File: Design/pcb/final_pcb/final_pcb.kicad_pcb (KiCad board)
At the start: 2 copper layers, 86.5 x 42 mm, 42 parts, among them J1 USB_C_Receptacle_USB2.0_14P, J2 Screw_Terminal_01x02, J3 Screw_Terminal_01x02, J5 Conn_01x05_Pin, Q1 NMOS, Q2 NMOS, U1 IR2184, U2 PIC32MZ2048EFM144-I/PH, U3 LM7812, U5 TPS560200, Y1 SG-8002CA

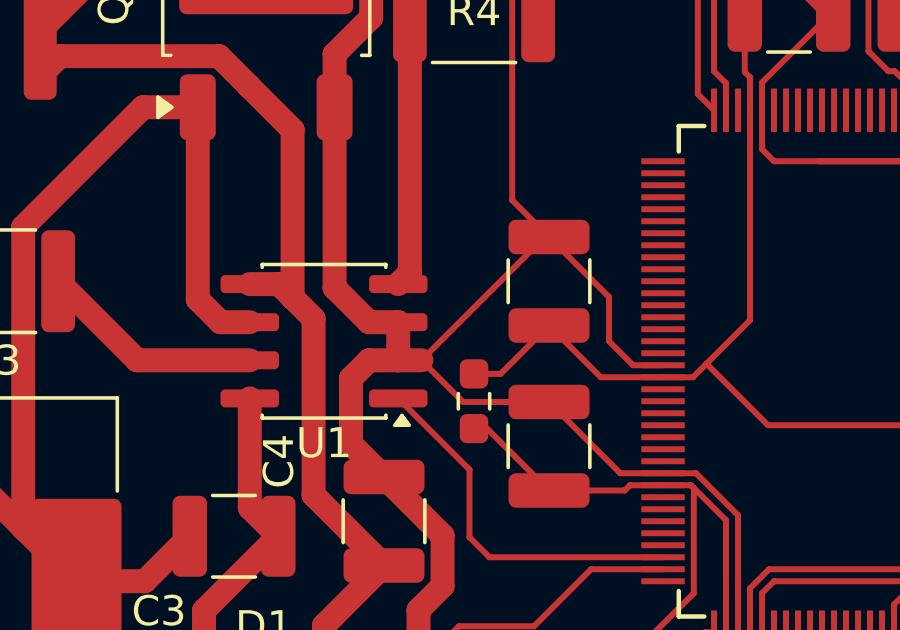
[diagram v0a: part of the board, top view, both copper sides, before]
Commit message: pcb fix
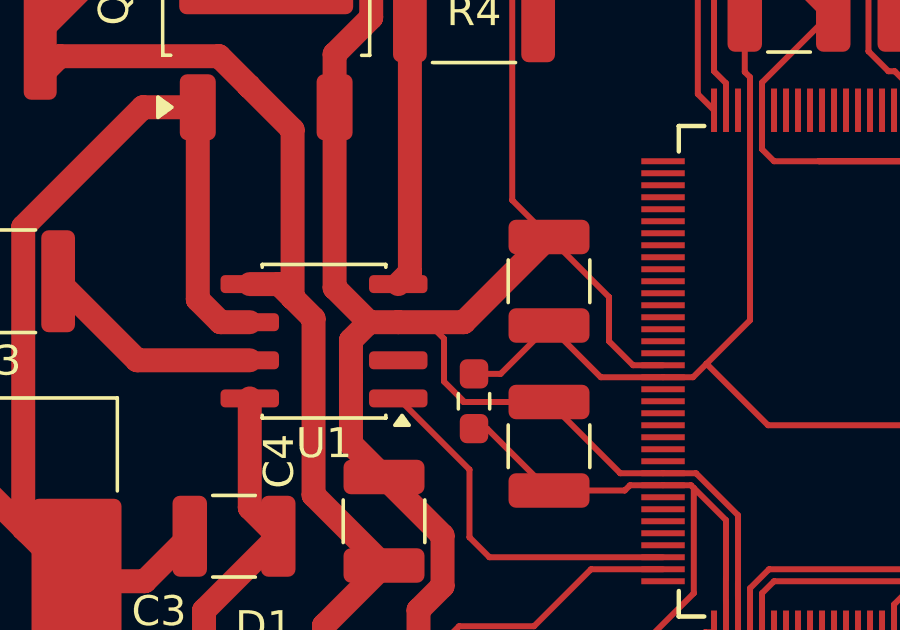
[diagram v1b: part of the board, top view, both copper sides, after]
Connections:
- U1 pad 2: GND -> unconnected-(U1-~{SD}-Pad2)
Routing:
- net GND: track 453.0 -> 454.1 mm
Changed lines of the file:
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@@
 	(net 143 "Net-(U5-FB)")
 	(net 144 "Net-(U5-PH)")
+	(net 145 "unconnected-(U1-~{SD}-Pad2)")
 	(footprint "Capacitor_SMD:C_1210_3225Metric"
 		(layer "F.Cu")
@@
 			(layers "F.Cu" "F.Mask" "F.Paste")
 			(roundrect_rratio 0.25)
-			(net 2 "GND")
+			(net 145 "unconnected-(U1-~{SD}-Pad2)")
 			(pinfunction "~{SD}")
 			(pintype "input")
@@
 	)
 	(segment
-		(start 113.246232 89.135)
-		(end 112.475 89.135)
-		(width 0.8)
-		(layer "F.Cu")
-		(net 2)
-	)
-	(segment
 		(start 142.434032 72.051)
 		(end 143.840968 72.051)
@@
 	)
 	(segment
+		(start 115 90.525)
+		(end 114.681866 90.525)
+		(width 0.2)
+		(layer "F.Cu")
+		(net 2)
+	)
+	(segment
 		(start 111.5735 73.789)
 		(end 112.8625 72.5)
@@
 	)
 	(segment
+		(start 110.899 89.736001)
+		(end 110.899 88.466001)
+		(width 0.8)
+		(layer "F.Cu")
+		(net 2)
+	)
+	(segment
 		(start 137.5 71.975)
 		(end 138.975 70.5)
@@
 	)
 	(segment
-		(start 117.356232 85.025)
-		(end 113.246232 89.135)
+		(start 114 89.843134)
+		(end 114 88.415001)
 		(width 0.2)
 		(layer "F.Cu")
@@
 	)
 	(segment
+		(start 114.66 87.865)
+		(end 117.5 85.025)
+		(width 0.8)
+		(layer "F.Cu")
+		(net 2)
+	)
+	(segment
 		(start 98 78.15)
 		(end 98 69)
@@
 	)
 	(segment
+		(start 113.449999 87.865)
+		(end 112.475 87.865)
+		(width 0.2)
+		(layer "F.Cu")
+		(net 2)
+	)
+	(segment
 		(start 116.274 83.799)
 		(end 116.274 75.9115)
@@
 	)
 	(segment
+		(start 114 88.415001)
+		(end 113.449999 87.865)
+		(width 0.2)
+		(layer "F.Cu")
+		(net 2)
+	)
+	(segment
 		(start 98 70.5)
 		(end 97 69.5)
@@
 	)
 	(segment
+		(start 110.899 88.466001)
+		(end 111.500001 87.865)
+		(width 0.8)
+		(layer "F.Cu")
+		(net 2)
+	)
+	(segment
 		(start 90.526 102.001)
 		(end 111.359424 102.001)
@@
 	)
 	(segment
-		(start 110.899 89.736001)
-		(end 111.500001 89.135)
-		(width 0.8)
-		(layer "F.Cu")
-		(net 2)
-	)
-	(segment
 		(start 123.8 99.3)
 		(end 124.975 100.475)
@@
 	)
 	(segment
-		(start 112.475 87.865)
-		(end 111.500001 87.865)
-		(width 0.8)
-		(layer "F.Cu")
-		(net 2)
-	)
-	(segment
 		(start 117.5 85.025)
 		(end 117.356232 85.025)
@@
 	)
 	(segment
-		(start 112.475 87.865)
-		(end 112.475 89.135)
-		(width 0.8)
-		(layer "F.Cu")
-		(net 2)
-	)
-	(segment
 		(start 146.5 82.3625)
 		(end 150.3675 82.3625)
@@
 	)
 	(segment
+		(start 115 90.525)
+		(end 114.636232 90.525)
+		(width 0.2)
+		(layer "F.Cu")
+		(net 2)
+	)
+	(segment
 		(start 98 69)
 		(end 80.828 69)
@@
 	)
 	(segment
+		(start 112.475 87.865)
+		(end 114.66 87.865)
+		(width 0.8)
+		(layer "F.Cu")
+		(net 2)
+	)
+	(segment
 		(start 138.975 101.5)
 		(end 138.975 100.175)
@@
 	)
 	(segment
+		(start 114.681866 90.525)
+		(end 114 89.843134)
+		(width 0.2)
+		(layer "F.Cu")
+		(net 2)
+	)
+	(segment
 		(start 110.3525 80.7)
 		(end 110.3525 78.930426)
@@
 	(segment
 		(start 117.5 90.525)
-		(end 114.636232 90.525)
+		(end 115 90.525)
 		(width 0.2)
 		(layer "F.Cu")
@@
 	)
 	(segment
+		(start 111.500001 87.865)
+		(end 112.475 87.865)
+		(width 0.8)
+		(layer "F.Cu")
+		(net 2)
+	)
+	(segment
 		(start 141.475 90.025)
 		(end 140.6 90.9)
@@
 	)
 	(segment
-		(start 111.500001 89.135)
-		(end 112.475 89.135)
-		(width 0.8)
-		(layer "F.Cu")
-		(net 2)
-	)
-	(segment
 		(start 150.725 78.1375)
 		(end 146.5 82.3625)
@@
 		(layer "F.Cu")
 		(net 2)
-	)
-	(segment
-		(start 114.636232 90.525)
-		(end 113.246232 89.135)
-		(width 0.2)
-		(layer "F.Cu")
-		(net 2)
